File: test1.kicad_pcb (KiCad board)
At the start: 2 copper layers, 35.6 x 71.1 mm, 22 parts, among them P1 Conn_01x03, P2 Conn_01x02, P3 Conn_01x04, U1 L78L05_TO92, U2 LM339

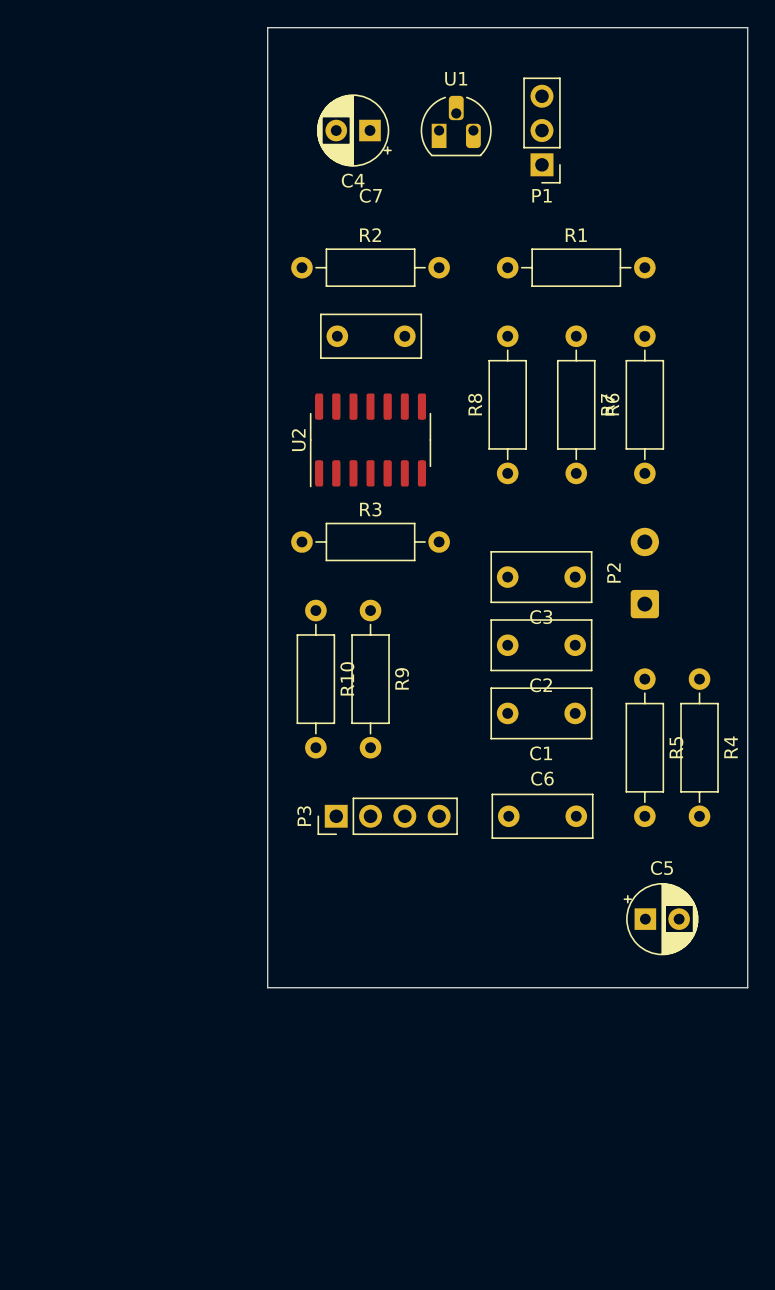
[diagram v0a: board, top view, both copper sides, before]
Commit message: dalawa nalang
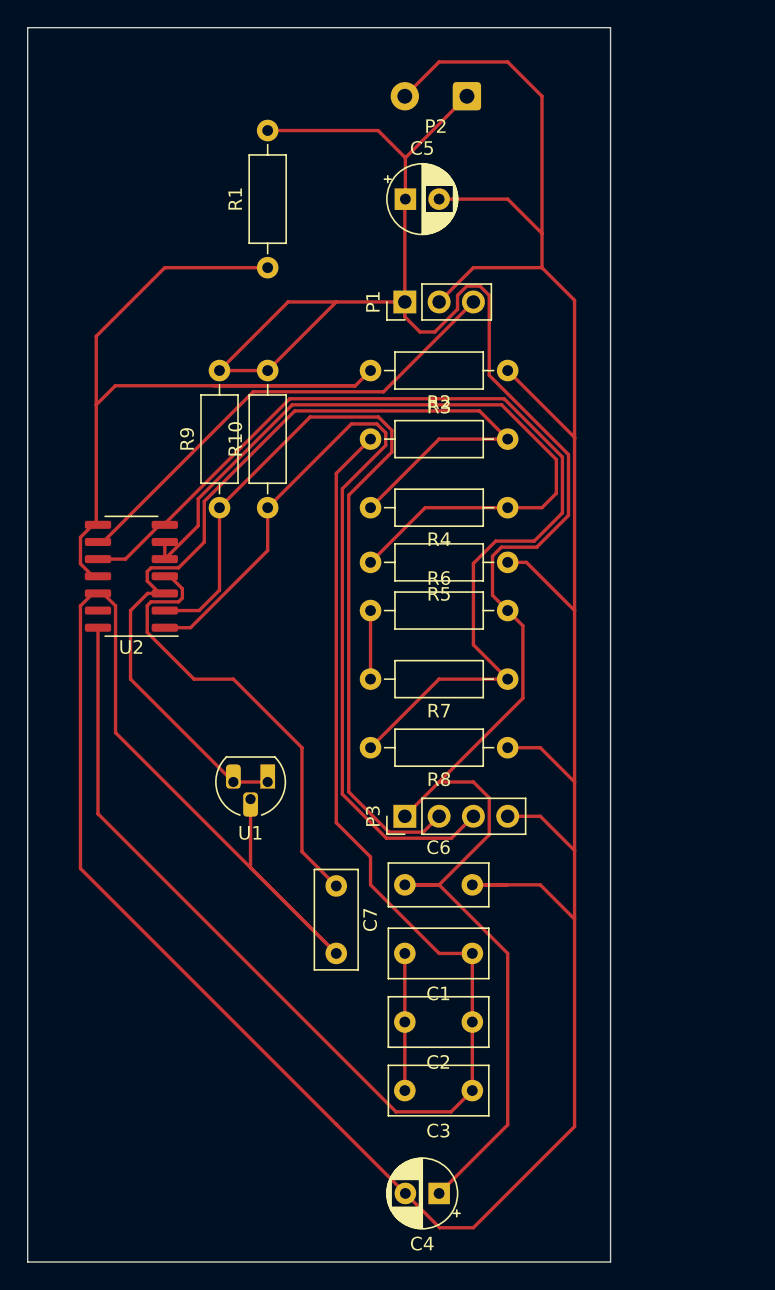
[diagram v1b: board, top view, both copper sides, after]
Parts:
- moved C4 78.9 mm to (165.1, 137.2)
- moved C5 56.2 mm to (162.6, 63.5)
- moved U1 49.9 mm to (152.4, 106.7), turned to 180 degrees
- moved C7 40.7 mm to (157.5, 114.4), turned to -90 degrees
- moved P2 39.9 mm to (167.2, 55.9), turned to 180 degrees
- moved C3 38.8 mm to (167.6, 129.5)
- moved C2 28.9 mm to (167.6, 124.5)
- moved R7 25.9 mm to (170.2, 99.1), turned to 180 degrees
- moved R6 22.7 mm to (160.0, 94.0), turned to 0 degrees
- moved U2 20.4 mm to (142.3, 91.4), turned to 180 degrees
- moved R8 20.3 mm to (170.2, 104.1), turned to 180 degrees
- moved C1 19.3 mm to (167.6, 119.4)
- moved R4 19.1 mm to (170.2, 86.4), turned to 180 degrees
- moved R1 17.8 mm to (152.4, 68.6), turned to 90 degrees
- moved R2 17.0 mm to (170.2, 76.2), turned to 180 degrees
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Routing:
- net GND: track 0.00 -> 263.9 mm
- net Net-(P1-Pin_1): track 0.00 -> 229.0 mm
- net Net-(C1-Pad1): track 0.00 -> 106.2 mm
- net Net-(U2B-+): track 0.00 -> 75.3 mm
- net Net-(U2A-+): track 0.00 -> 66.4 mm
- net Net-(U2C-+): track 0.00 -> 66.1 mm
- net Net-(P3-Pin_3): track 0.00 -> 64.6 mm
- net Net-(P3-Pin_2): track 0.00 -> 63.3 mm
- net Net-(U2A--): track 0.08 -> 38.6 mm
- net Net-(P1-Pin_3): track 0.00 -> 35.7 mm
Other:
- board size 35.6 x 71.1 mm -> 43.2 x 91.4 mm
